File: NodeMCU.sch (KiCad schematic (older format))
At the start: 1 part, among them U2 ESP-12E

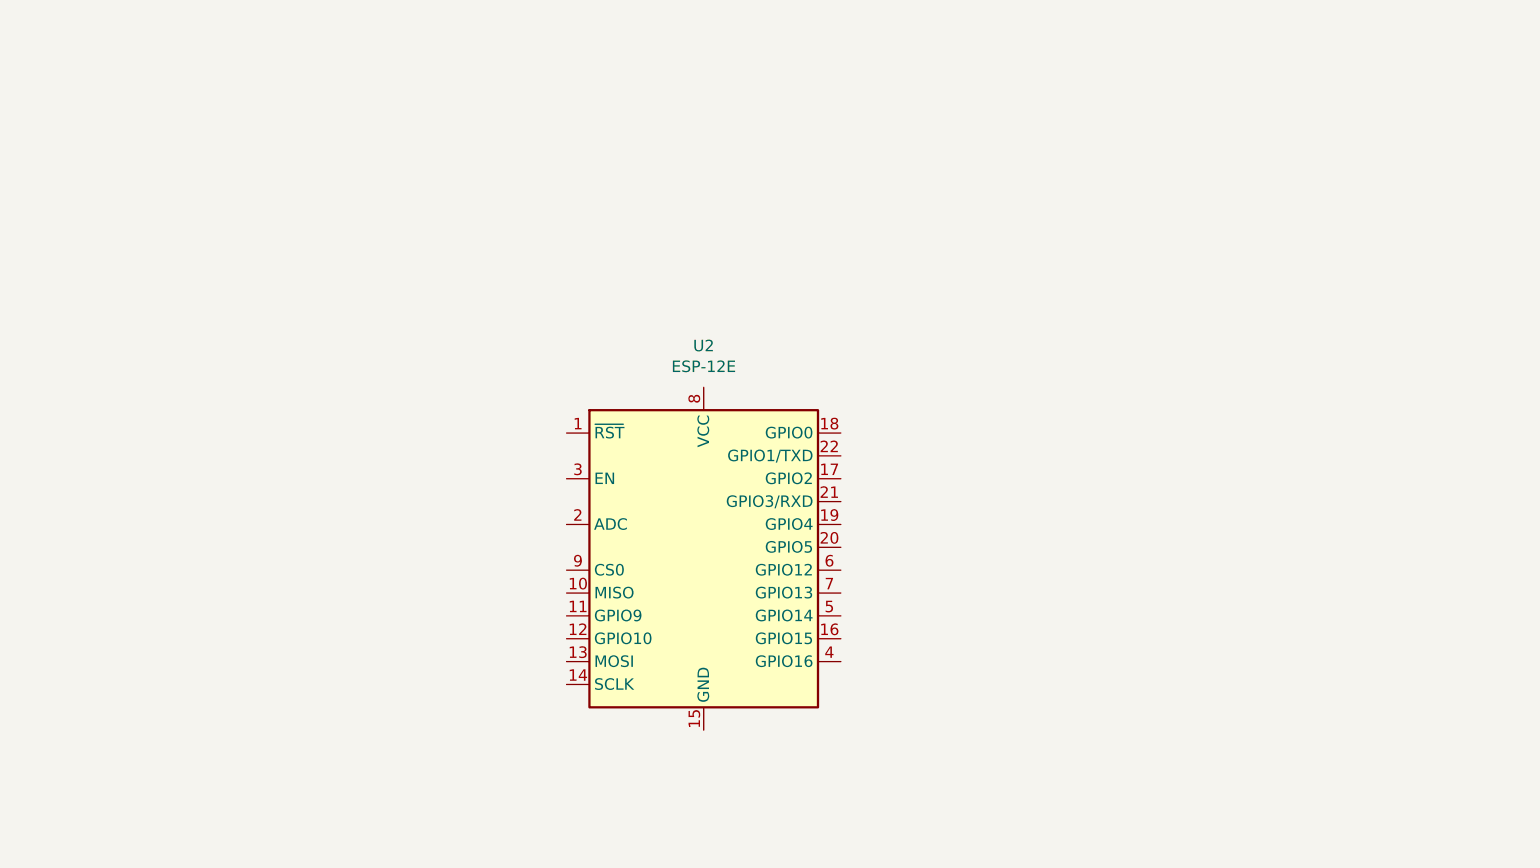
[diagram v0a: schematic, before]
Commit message: update files
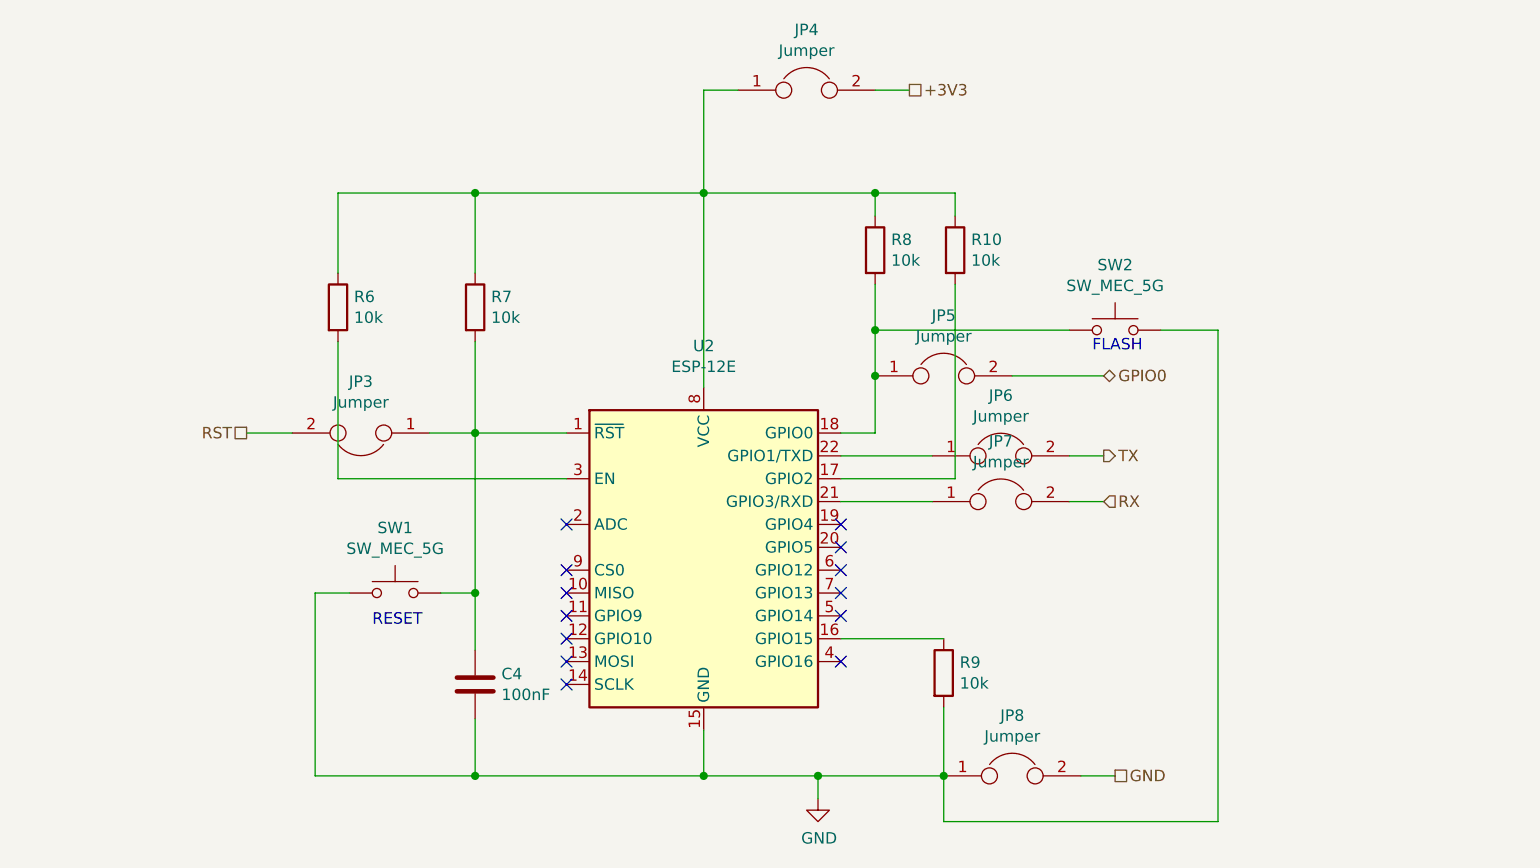
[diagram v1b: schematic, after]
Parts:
- added C4: 100nF, symbol Device:C
- added JP3, JP4, JP5, JP6, JP7, JP8: Jumper, Connector_PinHeader_2.54mm:PinHeader_1x02_P2.54mm_Vertical, symbol Device:Jumper
- added R10, R6, R7, R8, R9: 10k, Resistor_SMD:R_1206_3216Metric, symbol Device:R
- added SW1, SW2: SW_MEC_5G, Button_Switch_THT:SW_PUSH_6mm, symbol Switch:SW_MEC_5G
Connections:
- net at U2.1 (~RST): now also C4.1, JP3.1, R7.2, SW1.3 (B), SW1.4 (B)
- net GND: now reaches U2.15 (GND)
- net GND: now also C4.2, JP8.1, JP8.2, R9.2, SW1.1 (A), SW1.2 (A), SW2.3 (B), SW2.4 (B)
- net at U2.16 (GPIO15): now also R9.1
- net at U2.17 (GPIO2): now also R10.2
- net at U2.18 (GPIO0): now also JP5.1, R8.2, SW2.1 (A), SW2.2 (A)
- net at U2.21 (GPIO3/RXD): now also JP7.1
- net at U2.22 (GPIO1/TXD): now also JP6.1
- net at U2.3 (EN): now also R6.2
- net at U2.8 (VCC): now also JP4.1, R10.1, R6.1, R7.1, R8.1
- new net +3V3: JP4.2
- new net GPIO0: JP5.2
- new net RST: JP3.2
- new net RX: JP7.2
- new net TX: JP6.2
- no-connect marks 0 -> 13
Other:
- note added: "FLASH\n"
- note added: "RESET\n"

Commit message: update files
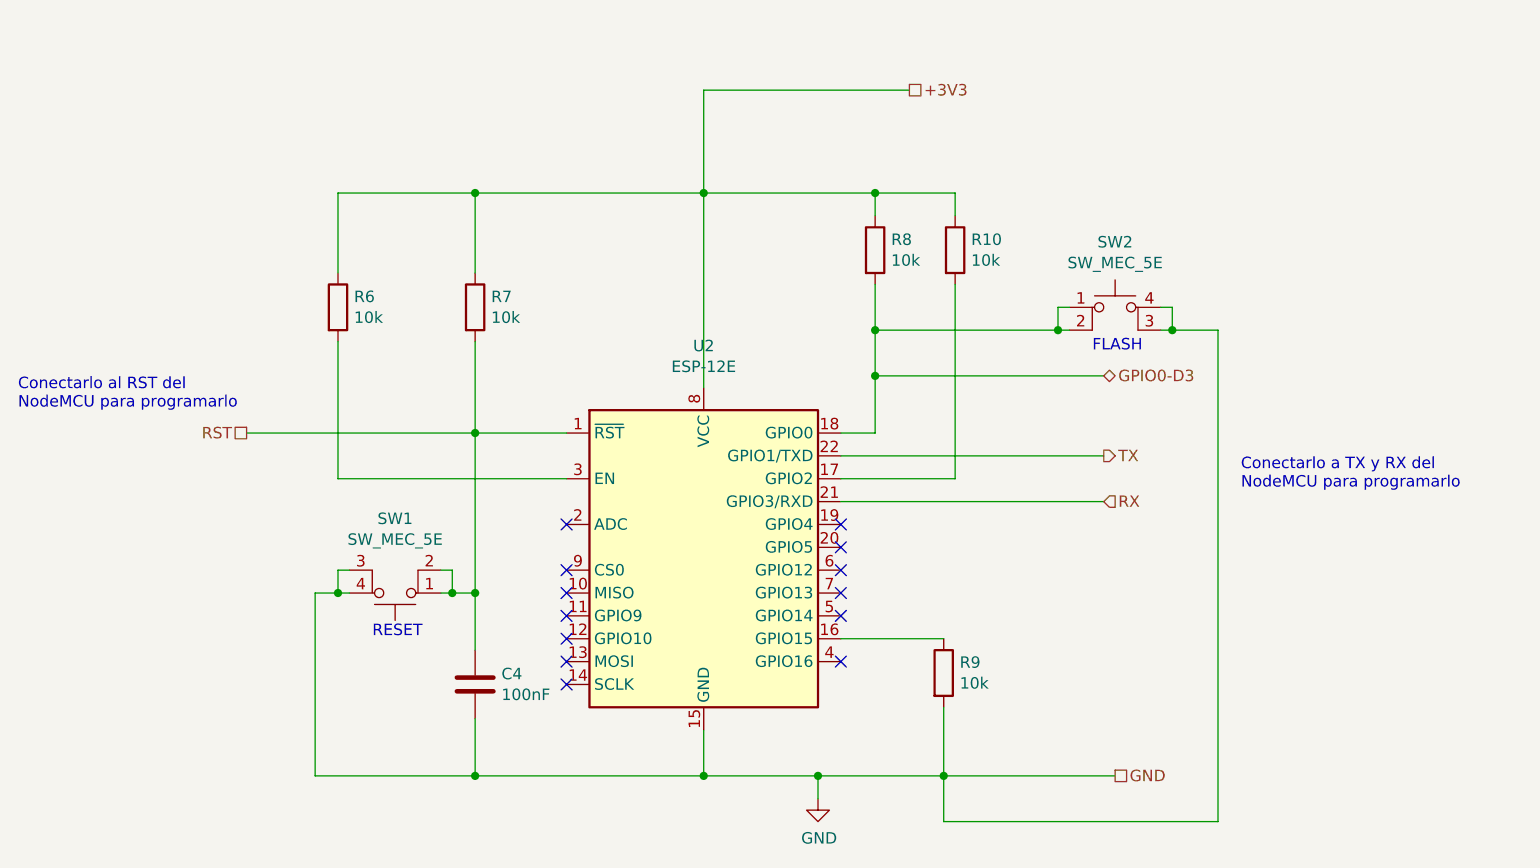
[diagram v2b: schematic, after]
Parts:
- removed JP3, JP4, JP5, JP6, JP7, JP8: Jumper, Connector_PinHeader_2.54mm:PinHeader_1x02_P2.54mm_Vertical, symbol Device:Jumper
- removed SW1, SW2: SW_MEC_5G, Button_Switch_THT:SW_PUSH_6mm, symbol Switch:SW_MEC_5G
- added SW1, SW2: SW_MEC_5E, Button_Switch_THT:SW_PUSH_6mm, symbol Switch:SW_MEC_5E
- C4: footprint (none) -> Capacitor_SMD:C_1206_3216Metric_Pad1.33x1.80mm_HandSolder
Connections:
- net +3V3: now also R10.1, R6.1, R7.1, R8.1, U2.8 (VCC)
- net GND: now also SW1.3 (K), SW1.4 (A), SW2.3 (K), SW2.4 (A)
- net RST: now also C4.1, R7.2, U2.1 (~RST), SW1.1, SW1.2
- net RX: now also U2.21 (GPIO3/RXD)
- net TX: now also U2.22 (GPIO1/TXD)
- net GPIO0-D3: now reaches R8.2, U2.18 (GPIO0)
- net GPIO0-D3: now also SW2.1, SW2.2
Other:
- note added: "Conectarlo a TX y RX del \nNodeMCU para programarlo"
- note added: "Conectarlo al RST del \nNodeMCU para programarlo"
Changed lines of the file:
@@
 Wire Wire Line
 	6250 3050 6100 3050
-Wire Wire Line
-	4300 3050 4500 3050
 Connection ~ 4500 3050
-$Comp
-L Device:Jumper JP3
-U 1 1 602A1CFC
-P 4000 3050
-F 0 "JP3" H 4000 2825 50  0000 C CNN
-F 1 "Jumper" H 4000 2916 50  0000 C CNN
-F 2 "Connector_PinHeader_2.54mm:PinHeader_1x02_P2.54mm_Vertical" H 4000 3050 50  0001 C CNN
-F 3 "~" H 4000 3050 50  0001 C CNN
-	1    4000 3050
-	-1   0    0    1
-$EndComp
 Wire Wire Line
 	3900 3250 4900 3250
 Text HLabel 3500 3050 0    50   UnSpc ~ 0
 RST
-$Comp
-L Device:Jumper JP8
-U 1 1 602A41EE
-P 6850 4550
-F 0 "JP8" H 6850 4814 50  0000 C CNN
-F 1 "Jumper" H 6850 4723 50  0000 C CNN
-F 2 "Connector_PinHeader_2.54mm:PinHeader_1x02_P2.54mm_Vertical" H 6850 4550 50  0001 C CNN
-F 3 "~" H 6850 4550 50  0001 C CNN
-	1    6850 4550
-	1    0    0    -1
-$EndComp
 Connection ~ 6550 4550
 Text HLabel 7300 4550 2    50   UnSpc ~ 0
 GND
-Wire Wire Line
-	7300 4550 7150 4550
-$Comp
-L Device:Jumper JP6
-U 1 1 602A4FFD
-P 6800 3150
-F 0 "JP6" H 6800 3414 50  0000 C CNN
-F 1 "Jumper" H 6800 3323 50  0000 C CNN
-F 2 "Connector_PinHeader_2.54mm:PinHeader_1x02_P2.54mm_Vertical" H 6800 3150 50  0001 C CNN
-F 3 "~" H 6800 3150 50  0001 C CNN
-	1    6800 3150
-	1    0    0    -1
-$EndComp
-$Comp
-L Device:Jumper JP7
-U 1 1 602A55FF
-P 6800 3350
-F 0 "JP7" H 6800 3614 50  0000 C CNN
-F 1 "Jumper" H 6800 3523 50  0000 C CNN
-F 2 "Connector_PinHeader_2.54mm:PinHeader_1x02_P2.54mm_Vertical" H 6800 3350 50  0001 C CNN
-F 3 "~" H 6800 3350 50  0001 C CNN
-	1    6800 3350
-	1    0    0    -1
-$EndComp
-Wire Wire Line
-	6100 3150 6500 3150
-Wire Wire Line
-	6500 3350 6100 3350
 Text HLabel 7250 3150 2    50   Output ~ 0
 TX
-Wire Wire Line
-	7250 3150 7100 3150
 Text HLabel 7250 3350 2    50   Input ~ 0
 RX
 Wire Wire Line
-	7250 3350 7100 3350
-Wire Wire Line
 	5500 2000 5500 2850
-$Comp
-L Device:Jumper JP5
-U 1 1 602AA9BE
-P 6550 2800
-F 0 "JP5" H 6550 3064 50  0000 C CNN
-F 1 "Jumper" H 6550 2973 50  0000 C CNN
-F 2 "Connector_PinHeader_2.54mm:PinHeader_1x02_P2.54mm_Vertical" H 6550 2800 50  0001 C CNN
-F 3 "~" H 6550 2800 50  0001 C CNN
-	1    6550 2800
-	1    0    0    -1
-$EndComp
-Connection ~ 6250 2800
-Wire Wire Line
-	6250 2800 6250 3050
 Text HLabel 7250 2800 2    50   BiDi ~ 0
-GPIO0
-Wire Wire Line
-	7250 2800 6850 2800
+GPIO0-D3
 NoConn ~ 4900 3450
 NoConn ~ 4900 3650
@@
 NoConn ~ 6100 3550
 NoConn ~ 6100 3450
-$Comp
-L Device:Jumper JP4
-U 1 1 602B56ED
-P 5950 1550
-F 0 "JP4" H 5950 1814 50  0000 C CNN
-F 1 "Jumper" H 5950 1723 50  0000 C CNN
-F 2 "Connector_PinHeader_2.54mm:PinHeader_1x02_P2.54mm_Vertical" H 5950 1550 50  0001 C CNN
-F 3 "~" H 5950 1550 50  0001 C CNN
-	1    5950 1550
-	1    0    0    -1
-$EndComp
-Wire Wire Line
-	6400 1550 6250 1550
-Wire Wire Line
-	5650 1550 5500 1550
 Wire Wire Line
 	5500 1550 5500 2000
-Wire Wire Line
-	3500 3050 3700 3050
 Wire Wire Line
 	3900 2000 4500 2000
@@
 Wire Wire Line
 	6250 2000 6600 2000
-$Comp
-L Switch:SW_MEC_5G SW1
-U 1 1 602D82D0
-P 4150 3750
-F 0 "SW1" H 4150 4035 50  0000 C CNN
-F 1 "SW_MEC_5G" H 4150 3944 50  0000 C CNN
-F 2 "Button_Switch_THT:SW_PUSH_6mm" H 4150 3950 50  0001 C CNN
-F 3 "http://www.apem.com/int/index.php?controller=attachment&id_attachment=488" H 4150 3950 50  0001 C CNN
-	1    4150 3750
-	1    0    0    -1
-$EndComp
 Connection ~ 5500 4550
 Wire Wire Line
 	5500 4550 6000 4550
 Wire Wire Line
-	4350 3750 4500 3750
+	4350 3750 4400 3750
 Wire Wire Line
 	4500 3050 4500 3750
 Wire Wire Line
-	3950 3750 3800 3750
+	3950 3750 3900 3750
 Wire Wire Line
 	3800 3750 3800 4550
@@
 F 0 "C4" H 4615 4196 50  0000 L CNN
 F 1 "100nF" H 4615 4105 50  0000 L CNN
-F 2 "" H 4538 4000 50  0001 C CNN
+F 2 "Capacitor_SMD:C_1206_3216Metric_Pad1.33x1.80mm_HandSolder" H 4538 4000 50  0001 C CNN
 F 3 "~" H 4500 4150 50  0001 C CNN
 	1    4500 4150
@@
 Wire Wire Line
 	4500 4550 5500 4550
-Text Notes 4050 3900 0    50   ~ 0
+Text Notes 4050 3950 0    50   ~ 0
 RESET\n
-$Comp
-L Switch:SW_MEC_5G SW2
-U 1 1 602DE06C
-P 7300 2600
-F 0 "SW2" H 7300 2885 50  0000 C CNN
-F 1 "SW_MEC_5G" H 7300 2794 50  0000 C CNN
-F 2 "Button_Switch_THT:SW_PUSH_6mm" H 7300 2800 50  0001 C CNN
-F 3 "http://www.apem.com/int/index.php?controller=attachment&id_attachment=488" H 7300 2800 50  0001 C CNN
-	1    7300 2600
-	1    0    0    -1
-$EndComp
-Wire Wire Line
-	7100 2600 6250 2600
 Connection ~ 6250 2600
-Wire Wire Line
-	6250 2600 6250 2800
-Wire Wire Line
-	7500 2600 7750 2600
 Wire Wire Line
 	7750 2600 7750 4750
@@
 Text Notes 7200 2700 0    50   ~ 0
 FLASH\n
+Text Notes 2500 2950 0    50   ~ 0
+Conectarlo al RST del \nNodeMCU para programarlo
+Text Notes 7850 3300 0    50   ~ 0
+Conectarlo a TX y RX del \nNodeMCU para programarlo
+Wire Wire Line
+	7500 2600 7550 2600
+Wire Wire Line
+	7100 2600 7050 2600
+$Comp
+L Switch:SW_MEC_5E SW2
+U 1 1 6053E81A
+P 7300 2600
+F 0 "SW2" H 7300 2985 50  0000 C CNN
+F 1 "SW_MEC_5E" H 7300 2894 50  0000 C CNN
+F 2 "Button_Switch_THT:SW_PUSH_6mm" H 7300 2900 50  0001 C CNN
+F 3 "http://www.apem.com/int/index.php?controller=attachment&id_attachment=1371" H 7300 2900 50  0001 C CNN
+	1    7300 2600
+	1    0    0    -1
+$EndComp
+Wire Wire Line
+	7100 2500 7050 2500
+Wire Wire Line
+	7050 2500 7050 2600
+Connection ~ 7050 2600
+Wire Wire Line
+	7050 2600 6250 2600
+Wire Wire Line
+	7500 2500 7550 2500
+Wire Wire Line
+	7550 2500 7550 2600
+Connection ~ 7550 2600
+Wire Wire Line
+	7550 2600 7750 2600
+$Comp
+L Switch:SW_MEC_5E SW1
+U 1 1 60540E1F
+P 4150 3650
+F 0 "SW1" H 4150 3425 50  0000 C CNN
+F 1 "SW_MEC_5E" H 4150 3516 50  0000 C CNN
+F 2 "Button_Switch_THT:SW_PUSH_6mm" H 4150 3950 50  0001 C CNN
+F 3 "http://www.apem.com/int/index.php?controller=attachment&id_attachment=1371" H 4150 3950 50  0001 C CNN
+	1    4150 3650
+	-1   0    0    1
+$EndComp
+Wire Wire Line
+	3950 3650 3900 3650
+Wire Wire Line
+	3900 3650 3900 3750
+Connection ~ 3900 3750
+Wire Wire Line
+	3900 3750 3800 3750
+Wire Wire Line
+	4350 3650 4400 3650
+Wire Wire Line
+	4400 3650 4400 3750
+Connection ~ 4400 3750
+Wire Wire Line
+	4400 3750 4500 3750
+Wire Wire Line
+	3500 3050 4500 3050
+Wire Wire Line
+	5500 1550 6400 1550
+Wire Wire Line
+	6550 4550 7300 4550
+Wire Wire Line
+	6100 3150 7250 3150
+Wire Wire Line
+	6100 3350 7250 3350
+Wire Wire Line
+	6250 2600 6250 2800
+Wire Wire Line
+	6250 2800 7250 2800
+Connection ~ 6250 2800
+Wire Wire Line
+	6250 2800 6250 3050
 $EndSCHEMATC
